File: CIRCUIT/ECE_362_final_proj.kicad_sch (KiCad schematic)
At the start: 44 parts, among them SW1 X_scale, SW2 BUTTON_CAPTURE, SW3 BUTTON_MODE, SW4 Y_scale, SW5 BOOTSEL, SW6 RESET, U2 Opamp_Quad, U3 RP2350_80QFN

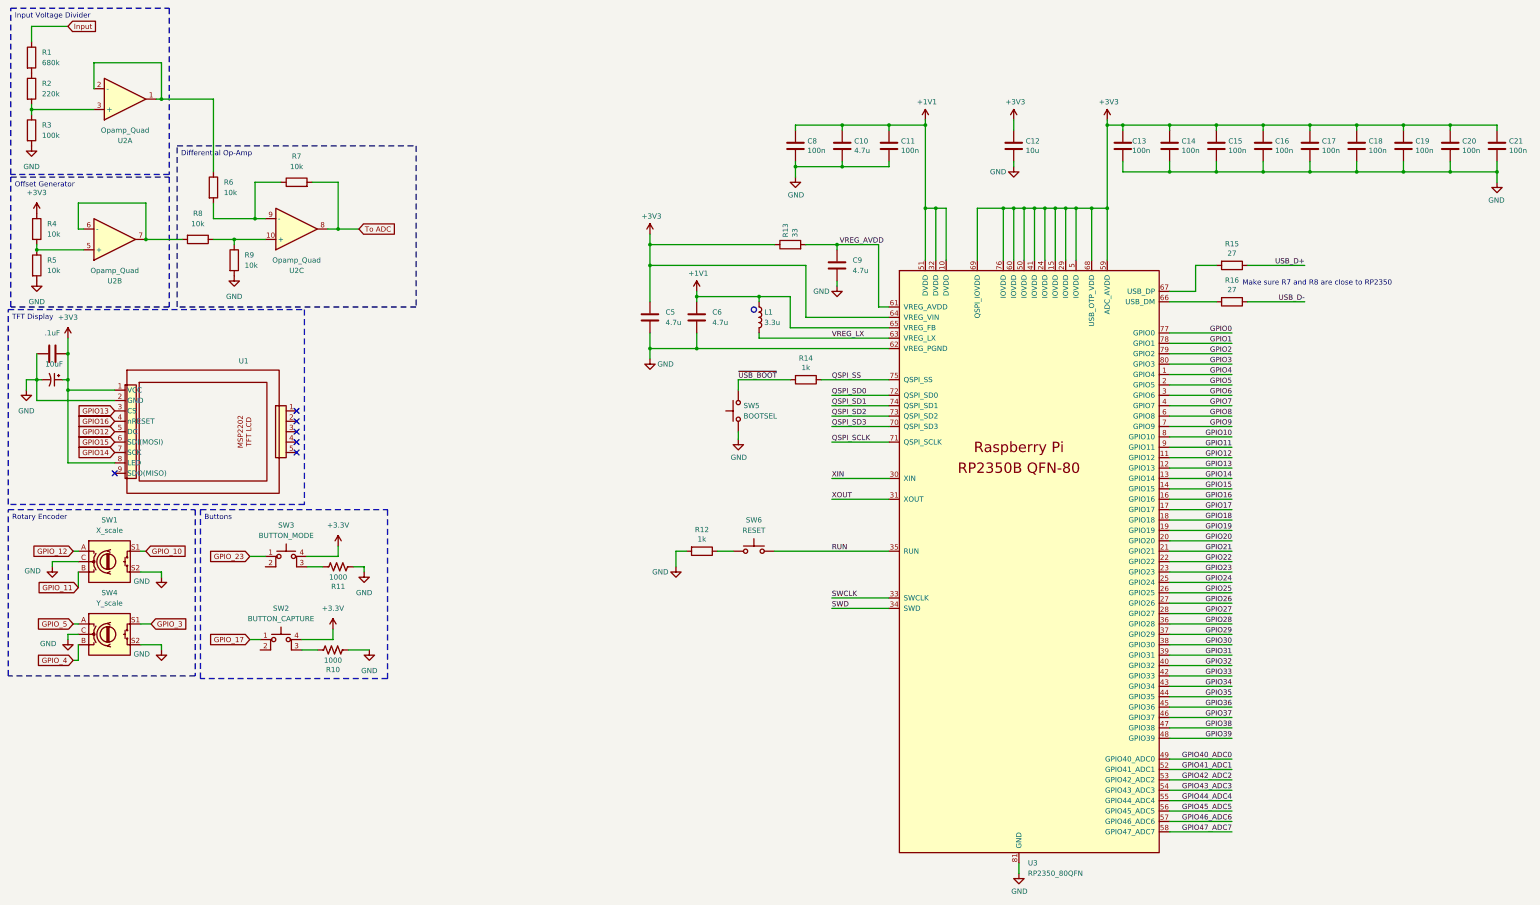
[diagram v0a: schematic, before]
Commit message: PCB lowkey done
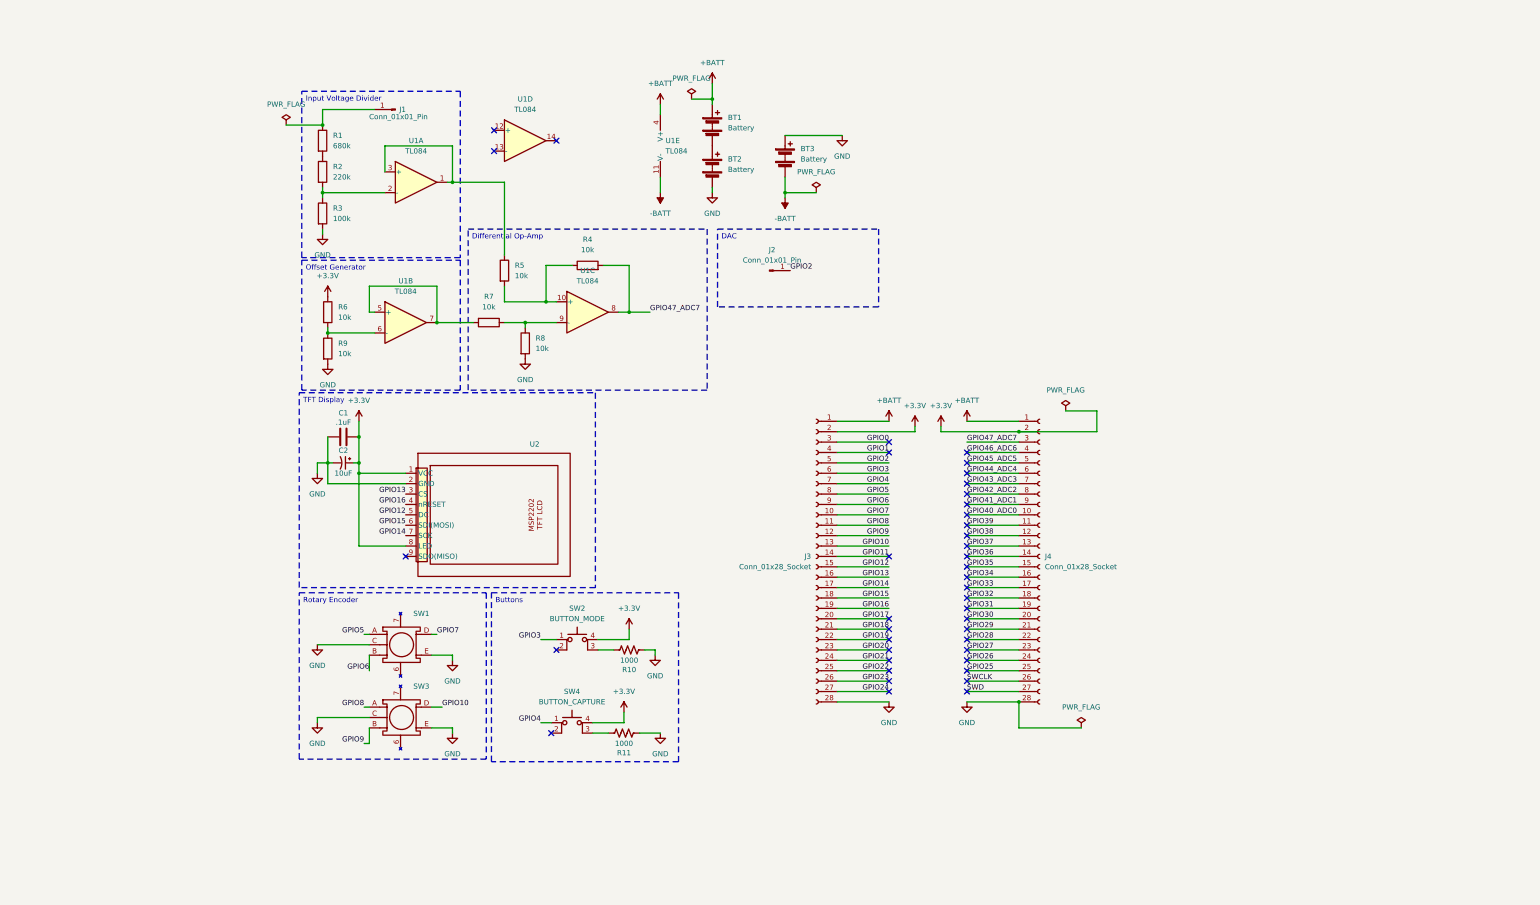
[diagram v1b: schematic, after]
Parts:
- removed C10, C9: 4.7u, Capacitor_SMD:C_0402_1005Metric, symbol Device:C
- removed C11, C13, C14, C15, C16, C17, C18, C19, C20, C21, C8: 100n, Capacitor_SMD:C_0402_1005Metric, symbol Device:C
- removed C12: 10u, Capacitor_SMD:C_0805_2012Metric, symbol Device:C
- removed C5, C6: 4.7u, RP2350_80QFN_minimal:C_0402_1005Metric_small_pads, symbol Device:C
- removed L1: 3.3u, RP2350_80QFN_minimal:L_pol_2016, symbol Device:L
- removed R12, R14: 1k, Resistor_SMD:R_0402_1005Metric, symbol Device:R
- removed R13: 33, Resistor_SMD:R_0402_1005Metric, symbol Device:R
- removed R15, R16: 27, Resistor_SMD:R_0402_1005Metric, symbol Device:R
- removed SW1: X_scale, symbol Device:RotaryEncoder_Switch
- removed SW4: Y_scale, symbol Device:RotaryEncoder_Switch
- removed SW5: BOOTSEL, Button_Switch_SMD:SW_SPST_PTS647_Sx38, symbol Switch:SW_Push
- removed SW6: RESET, Button_Switch_SMD:SW_SPST_PTS647_Sx38, symbol Switch:SW_Push
- removed U2: Opamp_Quad, symbol Device:Opamp_Quad
- removed U3: RP2350_80QFN, RP2350_80QFN_minimal:RP2350-QFN-80-1EP_10x10_P0.4mm_EP3.4x3.4mm_ThermalVias, symbol MCU_RaspberryPi_RP2350:RP2350_80QFN
- added BT1, BT2: Battery, cell_holder_3AA:BAT-TH_2P-L53.0-W24.6-P12.70_2468, symbol Device:Battery
- added BT3: Battery, cell_holder_3AA:BAT-TH_2479, symbol Device:Battery
- added J1, J2: Conn_01x01_Pin, Connector_PinHeader_2.00mm:PinHeader_1x01_P2.00mm_Vertical, symbol Connector:Conn_01x01_Pin
- added J3, J4: Conn_01x28_Socket, Connector_PinSocket_2.54mm:PinSocket_1x28_P2.54mm_Vertical, symbol Connector:Conn_01x28_Socket
- added SW1, SW3: ~, Rotary_Encoder_EC11E18244A5:SW-TH_EC11E18244A5, symbol Rotary_Encoder_EC11E18244A5:EC11E18244A5
- added U1: TL084, TL084:SOP-14_L8.6-W3.9-P1.27-LS6.0-BL, symbol Amplifier_Operational:TL084
- C1: footprint (none) -> Capacitor_SMD:C_0402_1005Metric
- C2: footprint (none) -> Capacitor_SMD:CP_Elec_4x4.5
- R1, R2, R3: footprint (none) -> Resistor_SMD:R_0402_1005Metric
- R10: renamed from R11; footprint (none) -> Resistor_SMD:R_0402_1005Metric
- R11: renamed from R10; footprint (none) -> Resistor_SMD:R_0402_1005Metric
- R4: renamed from R7; footprint (none) -> Resistor_SMD:R_0402_1005Metric
- R5: renamed from R6; footprint (none) -> Resistor_SMD:R_0402_1005Metric
- R6: renamed from R4; footprint (none) -> Resistor_SMD:R_0402_1005Metric
- R7: renamed from R8; footprint (none) -> Resistor_SMD:R_0402_1005Metric
- R8: renamed from R9; footprint (none) -> Resistor_SMD:R_0402_1005Metric
- R9: renamed from R5; footprint (none) -> Resistor_SMD:R_0402_1005Metric
- SW2: renamed from SW3; footprint (none) -> Button_Tactile:SW-TH_4P-L6.0-W6.0-P4.50-LS6.5
- SW4: renamed from SW2; footprint (none) -> Button_Tactile:SW-TH_4P-L6.0-W6.0-P4.50-LS6.5
- U2: renamed from U1; footprint (none) -> LCD_MSP2202_without_sd:LCD_MSP2202_without_sd
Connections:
- net +3V3 is gone; now on net +3.3V: C1.1, C2.1, R6.1, U2.1 (VCC), U2.8 (LED)
- net GPIO_17 is gone; now on net GPIO4: SW4.1
- net GPIO_23 is gone; now on net GPIO3: SW2.1
- net To ADC is gone; now on net GPIO47_ADC7: R4.2
- net +3.3V: now also J3.2 (Pin_2), J4.2 (Pin_2)
- net GND: now also BT2.2 (-), BT3.1 (+), J3.28 (Pin_28), J4.28 (Pin_28), SW1.C, SW1.E, SW3.C, SW3.E
- net GPIO0: now also J3.3 (Pin_3)
- net GPIO1: now also J3.4 (Pin_4)
- net GPIO10: now also J3.13 (Pin_13), SW3.D
- net GPIO11: now also J3.14 (Pin_14)
- net GPIO12: now also J3.15 (Pin_15)
- net GPIO13: now also J3.16 (Pin_16)
- net GPIO14: now also J3.17 (Pin_17)
- net GPIO15: now also J3.18 (Pin_18)
- net GPIO16: now also J3.19 (Pin_19)
- net GPIO17: now also J3.20 (Pin_20)
- net GPIO18: now also J3.21 (Pin_21)
- net GPIO19: now also J3.22 (Pin_22)
- net GPIO2: now also J2.1 (Pin_1), J3.5 (Pin_5)
- net GPIO20: now also J3.23 (Pin_23)
- net GPIO21: now also J3.24 (Pin_24)
- net GPIO22: now also J3.25 (Pin_25)
- net GPIO23: now also J3.26 (Pin_26)
- net GPIO24: now also J3.27 (Pin_27)
- net GPIO25: now also J4.25 (Pin_25)
- net GPIO26: now also J4.24 (Pin_24)
- net GPIO27: now also J4.23 (Pin_23)
- net GPIO28: now also J4.22 (Pin_22)
- net GPIO29: now also J4.21 (Pin_21)
- net GPIO3: now also J3.6 (Pin_6)
- net GPIO30: now also J4.20 (Pin_20)
- net GPIO31: now also J4.19 (Pin_19)
- net GPIO32: now also J4.18 (Pin_18)
- net GPIO33: now also J4.17 (Pin_17)
- net GPIO34: now also J4.16 (Pin_16)
- net GPIO35: now also J4.15 (Pin_15)
- net GPIO36: now also J4.14 (Pin_14)
- net GPIO37: now also J4.13 (Pin_13)
- net GPIO38: now also J4.12 (Pin_12)
- net GPIO39: now also J4.11 (Pin_11)
- net GPIO4: now also J3.7 (Pin_7)
- net GPIO40_ADC0: now also J4.10 (Pin_10)
- net GPIO41_ADC1: now also J4.9 (Pin_9)
- net GPIO42_ADC2: now also J4.8 (Pin_8)
- net GPIO43_ADC3: now also J4.7 (Pin_7)
- net GPIO44_ADC4: now also J4.6 (Pin_6)
- net GPIO45_ADC5: now also J4.5 (Pin_5)
- net GPIO46_ADC6: now also J4.4 (Pin_4)
- net GPIO47_ADC7: now also J4.3 (Pin_3), U1.8
- net GPIO5: now also J3.8 (Pin_8), SW1.A
- net GPIO6: now also J3.9 (Pin_9), SW1.B
- net GPIO7: now also J3.10 (Pin_10), SW1.D
- net GPIO8: now also J3.11 (Pin_11), SW3.A
- net GPIO9: now also J3.12 (Pin_12), SW3.B
- net SWCLK: now also J4.26 (Pin_26)
- net SWD: now also J4.27 (Pin_27)
- net at R2.2, R3.1: now also U1.2 (-)
- net at R6.2, R9.1: now also U1.6 (-)
- net at R7.1, R8.1: now also U1.9 (-)
- net at R5.1: now also U1.1, U1.3 (+)
- net at R4.1, R5.2: now also U1.10 (+)
- net at R7.2: now also U1.5 (+), U1.7
- net Input: no longer names the net of R1.1
- net Input: now also J1.1 (Pin_1)
- new net: BT1.2 (-), BT2.1 (+)
- new net +BATT: BT1.1 (+), J3.1 (Pin_1), J4.1 (Pin_1), U1.4 (V+)
- new net -BATT: BT3.2 (-), U1.11 (V-)
- no-connect marks 6 -> 41
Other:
- note removed: "Make sure R7 and R8 are close to RP2350"
- moved on the sheet: R1, R10, R11, R2, R3, R4, R5, R6, R7, R8, R9, SW2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

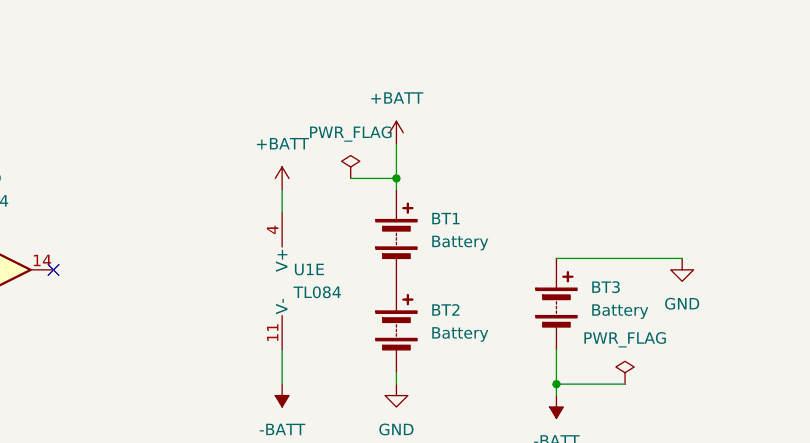
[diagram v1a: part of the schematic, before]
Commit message: rearranged board
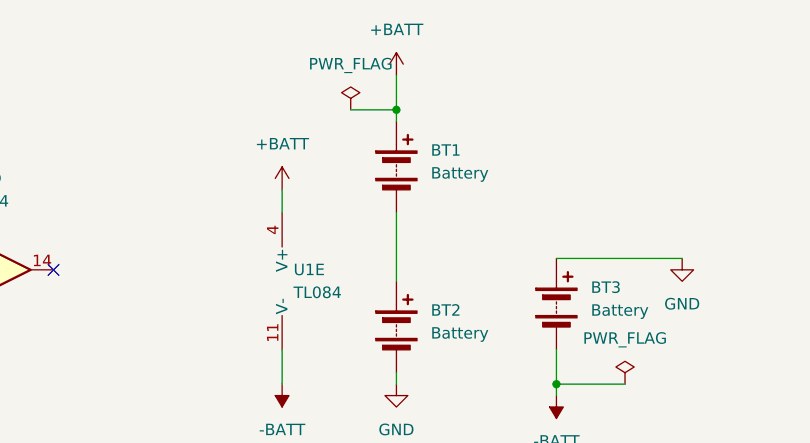
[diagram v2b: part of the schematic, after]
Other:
- moved on the sheet: BT1
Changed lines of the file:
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@@
 	)
 	(junction
-		(at 185.42 36.83)
+		(at 185.42 29.21)
 		(diameter 0)
 		(color 0 0 0 0)
@@
 	(wire
 		(pts
-			(xy 185.42 33.02) (xy 185.42 36.83)
+			(xy 185.42 25.4) (xy 185.42 29.21)
 		)
 		(stroke
@@
 	(wire
 		(pts
-			(xy 185.42 36.83) (xy 185.42 38.1)
+			(xy 185.42 29.21) (xy 185.42 30.48)
 		)
 		(stroke
@@
 	(wire
 		(pts
-			(xy 180.34 36.83) (xy 185.42 36.83)
+			(xy 180.34 29.21) (xy 185.42 29.21)
 		)
 		(stroke
@@
 	(wire
 		(pts
+			(xy 185.42 40.64) (xy 185.42 48.26)
+		)
+		(stroke
+			(width 0)
+			(type default)
+		)
+	)
+	(wire
+		(pts
 			(xy 228.6 140.97) (xy 215.9 140.97)
 		)
@@
 	(symbol
 		(lib_id "power:+BATT")
-		(at 185.42 33.02 0)
+		(at 185.42 25.4 0)
 		(unit 1)
 		(exclude_from_sim no)
@@
 		(fields_autoplaced yes)
 		(property "Reference" "#PWR01"
-			(at 185.42 36.83 0)
+			(at 185.42 29.21 0)
 			(effects
 				(font
@@
 		)
 		(property "Value" "+BATT"
-			(at 185.42 27.94 0)
+			(at 185.42 20.32 0)
 			(effects
 				(font
@@
 		)
 		(property "Footprint" ""
-			(at 185.42 33.02 0)
+			(at 185.42 25.4 0)
 			(effects
 				(font
@@
 		)
 		(property "Datasheet" ""
-			(at 185.42 33.02 0)
+			(at 185.42 25.4 0)
 			(effects
 				(font
@@
 		)
 		(property "Description" "Power symbol creates a global label with name \"+BATT\""
-			(at 185.42 33.02 0)
+			(at 185.42 25.4 0)
 			(effects
 				(font
@@
 	(symbol
 		(lib_id "power:PWR_FLAG")
-		(at 180.34 36.83 0)
+		(at 180.34 29.21 0)
 		(unit 1)
 		(exclude_from_sim no)
@@
 		(fields_autoplaced yes)
 		(property "Reference" "#FLG01"
-			(at 180.34 34.925 0)
+			(at 180.34 27.305 0)
 			(effects
 				(font
@@
 		)
 		(property "Value" "PWR_FLAG"
-			(at 180.34 31.75 0)
+			(at 180.34 24.13 0)
 			(effects
 				(font
@@
 		)
 		(property "Footprint" ""
-			(at 180.34 36.83 0)
+			(at 180.34 29.21 0)
 			(effects
 				(font
@@
 		)
 		(property "Datasheet" "~"
-			(at 180.34 36.83 0)
+			(at 180.34 29.21 0)
 			(effects
 				(font
@@
 		)
 		(property "Description" "Special symbol for telling ERC where power comes from"
-			(at 180.34 36.83 0)
+			(at 180.34 29.21 0)
 			(effects
 				(font
@@
 	(symbol
 		(lib_id "Device:Battery")
-		(at 185.42 43.18 0)
+		(at 185.42 35.56 0)
 		(unit 1)
 		(exclude_from_sim no)
@@
 		(fields_autoplaced yes)
 		(property "Reference" "BT1"
-			(at 189.23 41.3384 0)
+			(at 189.23 33.7184 0)
 			(effects
 				(font
@@
 		)
 		(property "Value" "Battery"
-			(at 189.23 43.8784 0)
+			(at 189.23 36.2584 0)
 			(effects
 				(font
@@
 		)
 		(property "Footprint" "cell_holder_3AA:BAT-TH_2P-L53.0-W24.6-P12.70_2468"
-			(at 185.42 41.656 90)
+			(at 185.42 34.036 90)
 			(effects
 				(font
@@
 		)
 		(property "Datasheet" "~"
-			(at 185.42 41.656 90)
+			(at 185.42 34.036 90)
 			(effects
 				(font
@@
 		)
 		(property "Description" "Multiple-cell battery - 4 cells"
-			(at 185.42 43.18 0)
+			(at 185.42 35.56 0)
 			(effects
 				(font
